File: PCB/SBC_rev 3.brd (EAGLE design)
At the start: 76.2 x 76.2 mm, 47 parts, among them IC1 74ALS00D, IC2 74LS138D, IC4 PCA9534D, IC5 PCA9534D, IC6 PCA9534D, IC7 74LS32D

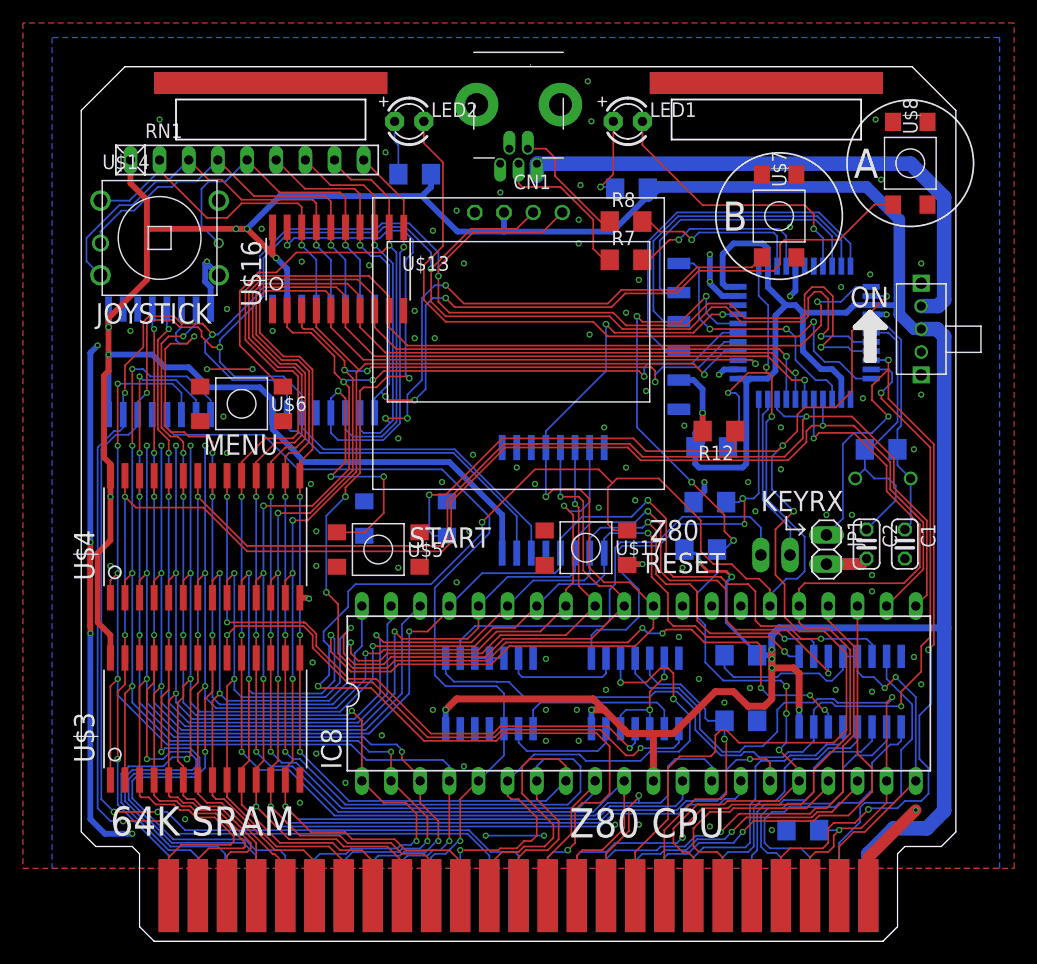
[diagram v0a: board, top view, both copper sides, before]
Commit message: Updates
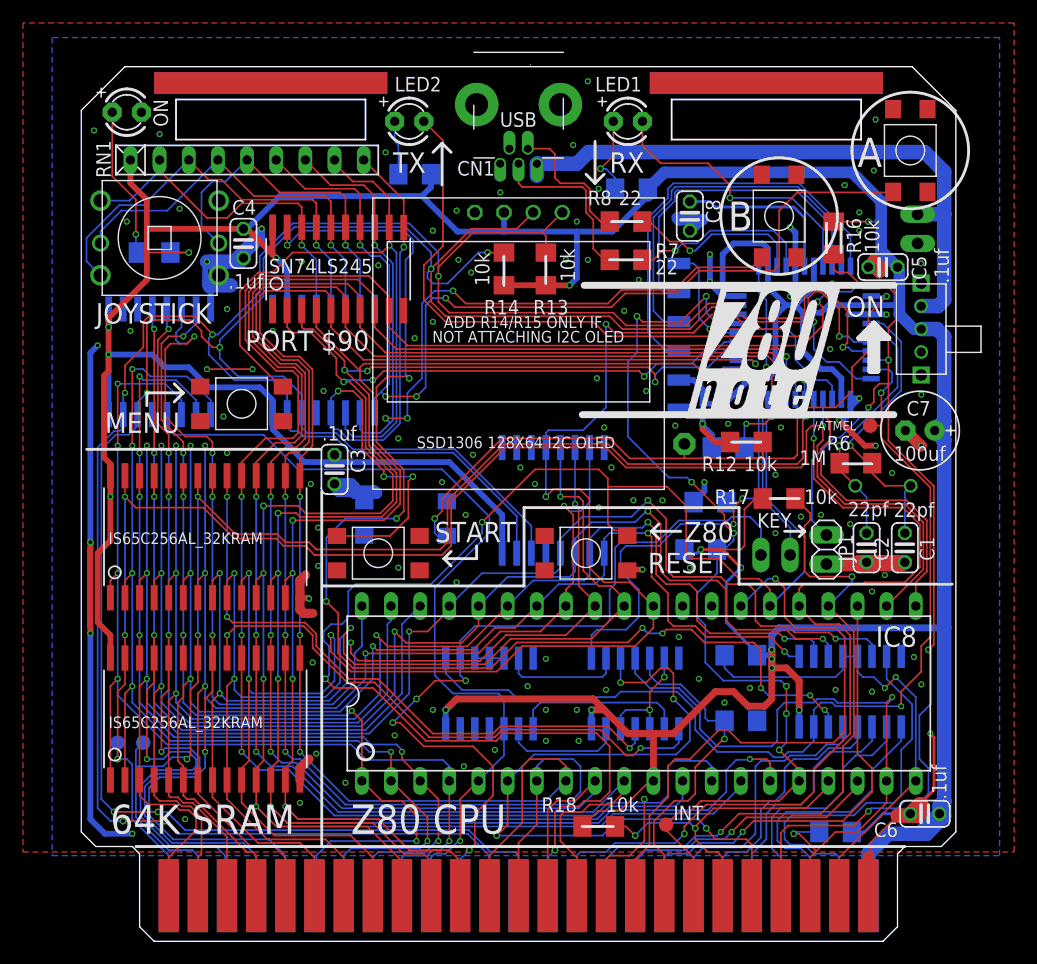
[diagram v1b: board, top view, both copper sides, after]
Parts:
- added /ATMEL, INT, RD, WR: TPB1,27, testpad:B1,27
- added C3, C4, C5, C6: .1uf, zx_kit2:RESISTOR_C025-024X044
- added C7: 100uf, adafruit:E2,5-7
- added C8: 1uf, zx_kit2:RESISTOR_C025-024X044
- added JP3: (no value), pinhead:1X02/90
- added ON: (no value), adafruit:LED3MM
- added R13, R14, R16, R17, R18: 10k, rcl:R1206
- added R15: 1k, rcl:R1206
- added RST: PROG, adafruit:1X01
- added SD_ADAPTER: SD_ADAPTER, OLED SSD1306 display:SD_RIGHTANGLE
- JP1: value KEYRX -> KEY
- JP2: value EXTCLK -> FASTCLK
- U$15: value SD_ADAPTER -> (none); device OLED SSD1306 display:SD_RIGHTANGLE -> 8-bit_computer:Z80LOGO
- moved U$15 7.17 mm to (52.7, 45.6), flipped to the top, turned to 0 degrees
- moved R4 2.86 mm to (65.7, 9.53), turned to 0 degrees
- moved R12 2.56 mm to (57.9, 43.5)
- moved R6 2.51 mm to (67.5, 41.7), flipped to the top, turned to 0 degrees
- moved R11 1.43 mm to (56.4, 43.0)
- moved U$8 1.11 mm to (72.2, 68.9)
- moved Q1 0.63 mm to (69.8, 39.7)
- moved U$17 0.48 mm to (44.0, 33.8)
- moved C1 0.32 mm to (71.8, 34.3)
- moved C2 0.32 mm to (68.4, 34.3)
- moved U$5 0.32 mm to (25.9, 33.8)
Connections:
- removed net N$27: IC8.27
- removed net N$3: U$1.P$41
- removed net _MCU_VBUS: U$2.7
- new net M1: IC8.27, U$1.P$33
- new net N$1: IC1.12
- new net N$2: IC1.13
- new net N$7: ON.A, R15.2
- new net TIMER4: JP2.1, U$2.32
- net /ATMELSERIAL: now also /ATMEL.TP
- net /SDCS: now also SD_ADAPTER.P$6; no longer U$15.P$6
- net FASTCLK: now also IC1.2, JP2.2, U$1.P$22; no longer JP2.1, U$2.32
- net GND: now also C3.2, C4.2, C5.2, C6.2, C7.-, C8.2, JP3.2, ON.K, SD_ADAPTER.P$1; no longer U$15.P$1
- net INT: now also INT.TP
- net KEYBOARD_RX: now also R16.1
- net MCU_RST: now also RST.1; no longer U$1.P$33
- net MISO: now also SD_ADAPTER.P$3; no longer U$15.P$3
- net MOSI: now also SD_ADAPTER.P$4; no longer U$15.P$4
- net N$6: now also IC1.11; no longer IC1.2, JP2.2
- net NMI: now also R18.1
- net RD: now also RD.TP
- net SCK: now also SD_ADAPTER.P$5; no longer U$15.P$5
- net SCL: now also R14.1
- net SDA: now also R13.1
- net UCAP: now also C8.1
- net VBUS: now also JP3.1
- net VCC: now also C3.1, C4.1, C5.1, C6.1, C7.+, R13.2, R14.2, R15.1, R16.2, R17.2, R18.2, SD_ADAPTER.P$2, U$2.7; no longer U$15.P$2
- net WAIT: now also R17.1
- net WR: now also WR.TP
- net Z80CLK: now also U$1.P$41; no longer U$1.P$22
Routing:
- net GND: track 93.9 -> 186.3 mm, vias 105 -> 114
- net MCU_RST: track 121.3 -> 62.6 mm, vias 4 -> 2
- net FASTCLK: track 14.8 -> 71.2 mm, vias 0 -> 4
- net M1: track 0.00 -> 51.9 mm, vias 0 -> 1
- net VCC: track 404.6 -> 445.3 mm, vias 15 -> 16
- net N$6: track 38.4 -> 0.00 mm
- net Z80CLK: track 49.0 -> 64.7 mm, vias 3 -> 4
- net WAIT: track 43.8 -> 58.7 mm, vias 1 -> 2
- net UCAP: track 0.00 -> 14.8 mm
- net TIMER4: track 0.00 -> 14.8 mm
- net N$7: track 0.00 -> 13.2 mm, vias 0 -> 1
- net KEYBOARD_RX: track 80.0 -> 92.5 mm
- net $F0: track 25.9 -> 34.8 mm
- net NMI: track 21.6 -> 29.0 mm, vias 0 -> 2
- net SCL: track 220.2 -> 227.5 mm, vias 6 -> 7
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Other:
- board text added: "/SDCS"
- board text added: "16MHZ"
- board text added: "3:8 MUX"
- board text added: "5VDC"
- board text added: "ADD R14/R15 ONLY IF"
- board text added: "AUXPOW"
- board text added: "GND"
- board text added: "ICSP"
- board text added: "MCU RESET"
- board text added: "MISO"
- board text added: "MOSI"
- board text added: "NAND"
- board text added: "NOT ATTACHING I2C OLED"
- board text added: "OR"
- board text added: "PORT $90"
- board text added: "RX"
- board text added: "SCK"
- board text added: "SIDE"
- board text added: "SOLDER"
- board text added: "SSD1306 128X64 I2C OLED"
- board text added: "TIMER4"
- board text added: "TX"
- board text added: "USB"
- board text added: "VCC"
- board text added: "WWW.BENHECK.COM"
- board text removed: "KEYRX"
